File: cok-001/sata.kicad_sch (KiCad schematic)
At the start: 56 parts, among them J3401 Conn_01x22_Pin, Q3401 DTC144E, Q3404 DTC144E

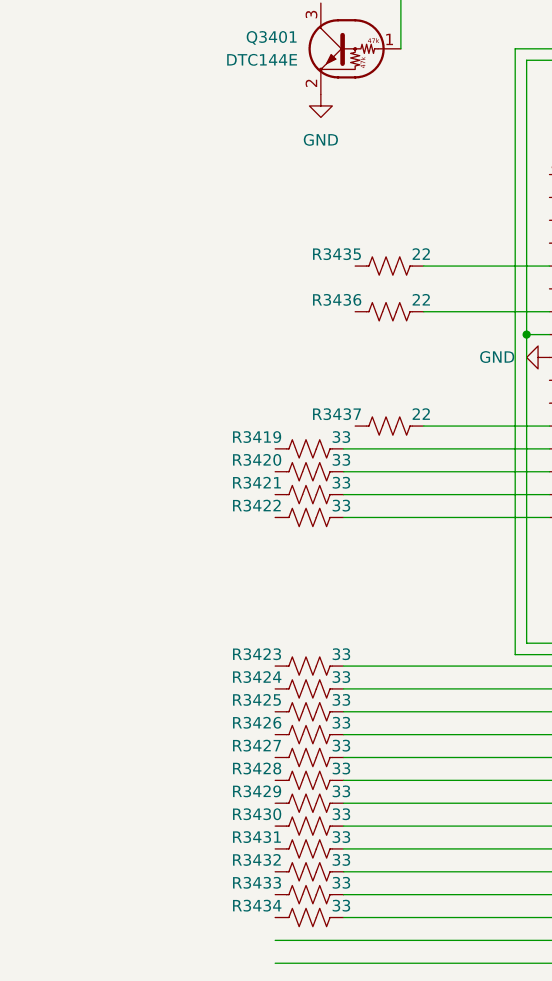
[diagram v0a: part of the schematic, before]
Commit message: southbridge
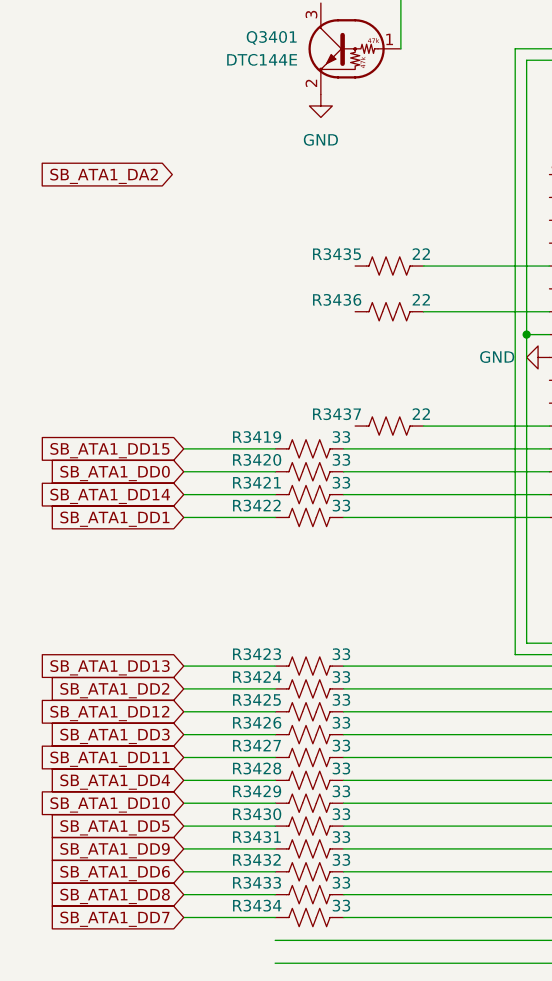
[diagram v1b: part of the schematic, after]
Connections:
- net SB_ATA1_DD12: now reaches R3425.1
- net SB_ATA1_DD10: now reaches R3429.1
- net SB_ATA1_DD13: now reaches R3423.1
- net SB_ATA1_DD11: now reaches R3427.1
- net SB_ATA1_DD0: now reaches R3420.1
- net SB_ATA1_DD7: now reaches R3434.1
- net SB_ATA1_DD3: now reaches R3426.1
- net SB_ATA1_DD1: now reaches R3422.1
- net SB_ATA1_DD14: now reaches R3421.1
- net SB_ATA1_DD5: now reaches R3430.1
- net SB_ATA1_DD15: now reaches R3419.1
- net SB_ATA1_DD8: now reaches R3433.1
- net SB_ATA1_DD2: now reaches R3424.1
- net SB_ATA1_DD9: now reaches R3431.1
- net SB_ATA1_DD6: now reaches R3432.1
- net SB_ATA1_DD4: now reaches R3428.1
